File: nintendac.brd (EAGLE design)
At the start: 43 x 43 mm, 35 parts, among them IC2 REG1117, U1 STM32F10XRXT6, X1 USB-MICROB

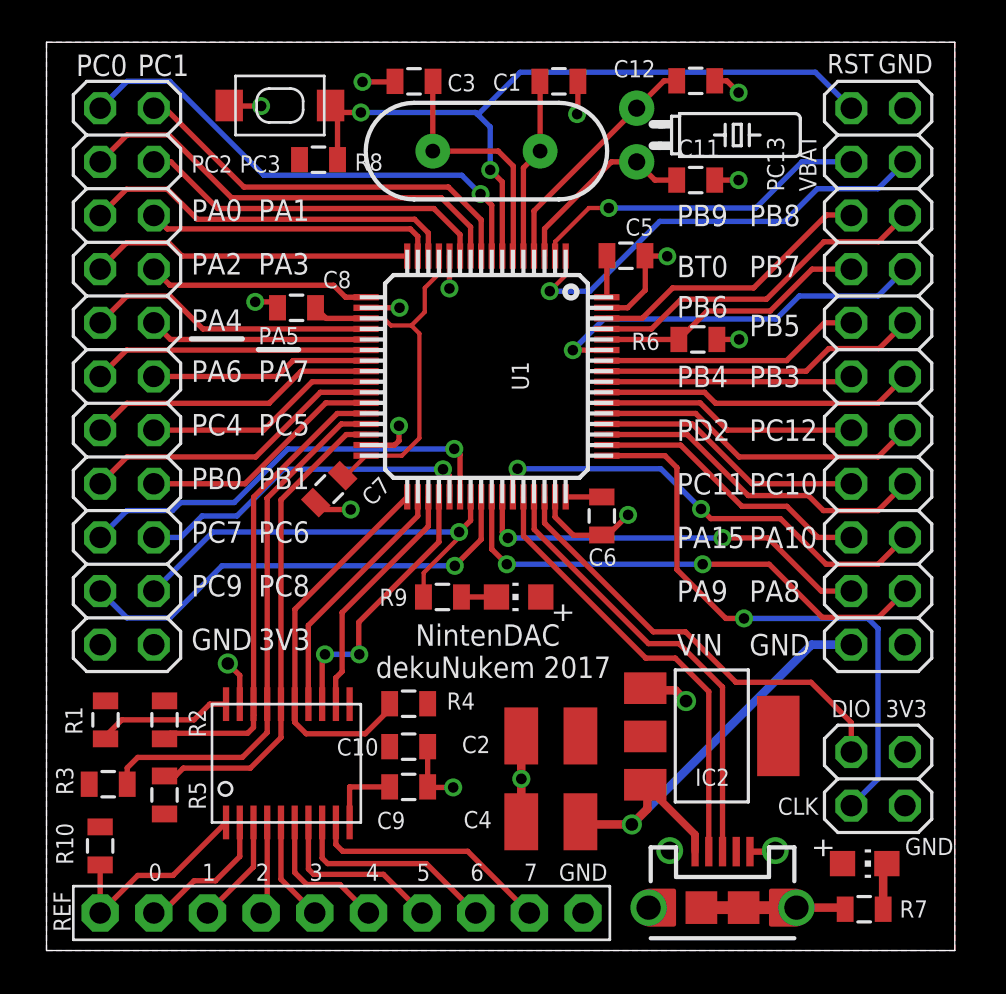
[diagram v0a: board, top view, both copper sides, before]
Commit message: board cleanup
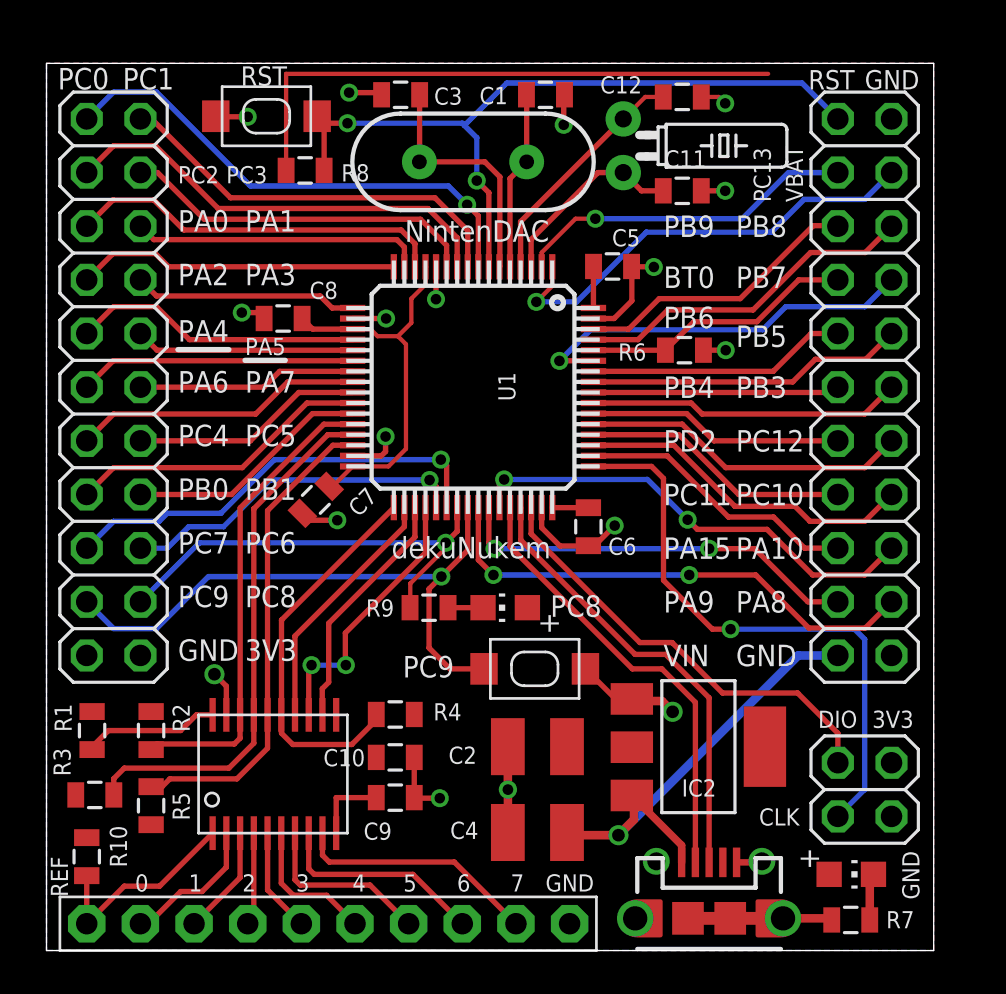
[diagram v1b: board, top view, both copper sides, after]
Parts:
- added S2: SWITCH-MOMENTARY-2TURTLE, Adafruit Feather M0 Adalogger:KMR2
- moved C12 0.99 mm to (30.1, 40.4)
- moved C1 0.90 mm to (23.6, 40.5)
- moved C3 0.90 mm to (16.8, 40.5)
- moved R7 0.81 mm to (38.1, 1.45)
- moved C11 0.81 mm to (30.1, 36.0)
- moved C6 0.81 mm to (25.7, 20.1)
- moved LED2 0.81 mm to (21.7, 16.2)
- moved R9 0.81 mm to (18.1, 16.2)
- moved C2 0.81 mm to (23.2, 9.65)
- moved C7 0.81 mm to (12.8, 21.3)
- moved C8 0.81 mm to (11.2, 29.9)
- moved S1 0.81 mm to (10.4, 39.5)
- moved C4 0.81 mm to (23.2, 5.59)
- moved R1 0.81 mm to (2.16, 10.4)
- moved R2 0.81 mm to (4.95, 10.4)
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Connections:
- net GND: now also S2.1
- net N$30: now also S2.3
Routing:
- net +3V3: track 25.8 -> 53.2 mm
- net N$30: track 22.1 -> 28.8 mm
- net GND: track 46.5 -> 49.1 mm
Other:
- board size 43 x 43 mm -> 42 x 42 mm
- board text added: "dekuNukem"
- board text removed: "dekuNukem 2017"
